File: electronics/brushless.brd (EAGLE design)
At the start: 34.3 x 56.2 mm, 63 parts, among them J1 USB_MINI-B_SMT, X1 JST-XH-10-PIN-LONG-PAD

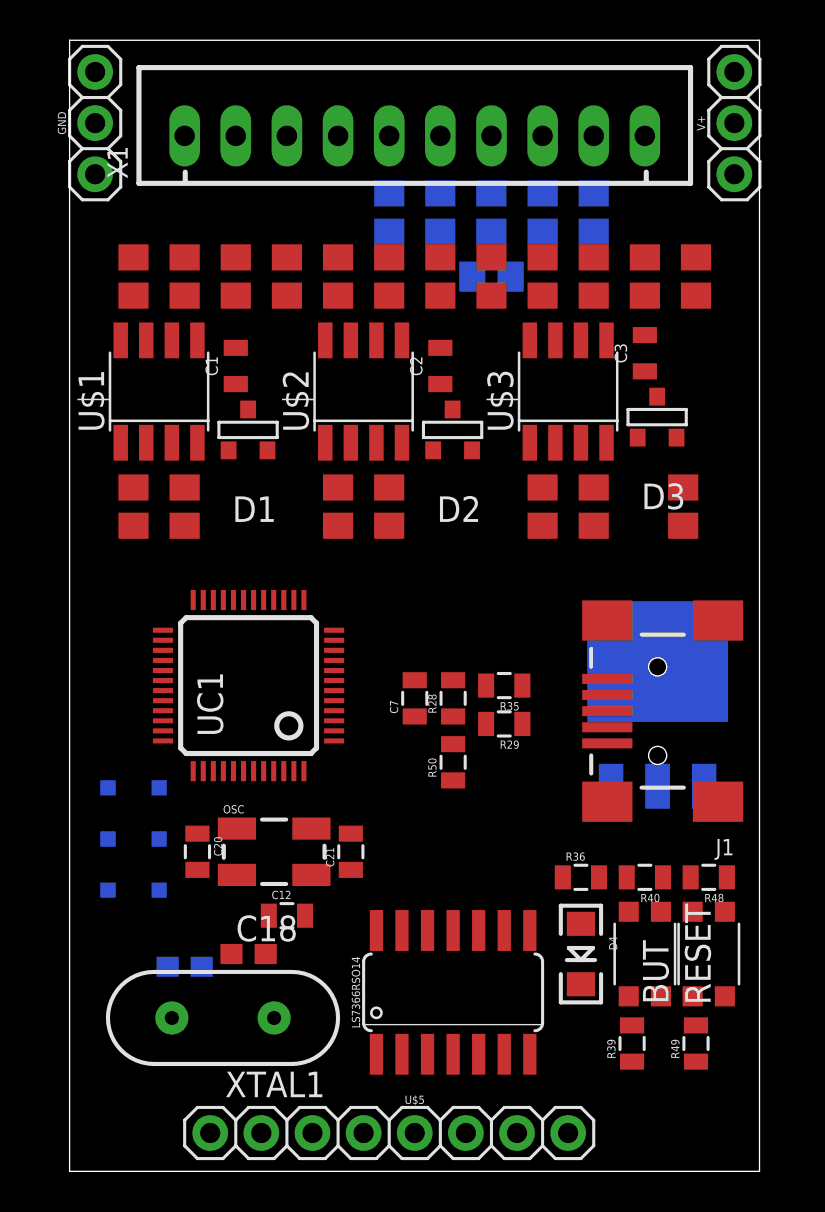
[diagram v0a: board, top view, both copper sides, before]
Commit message: mos (wip)
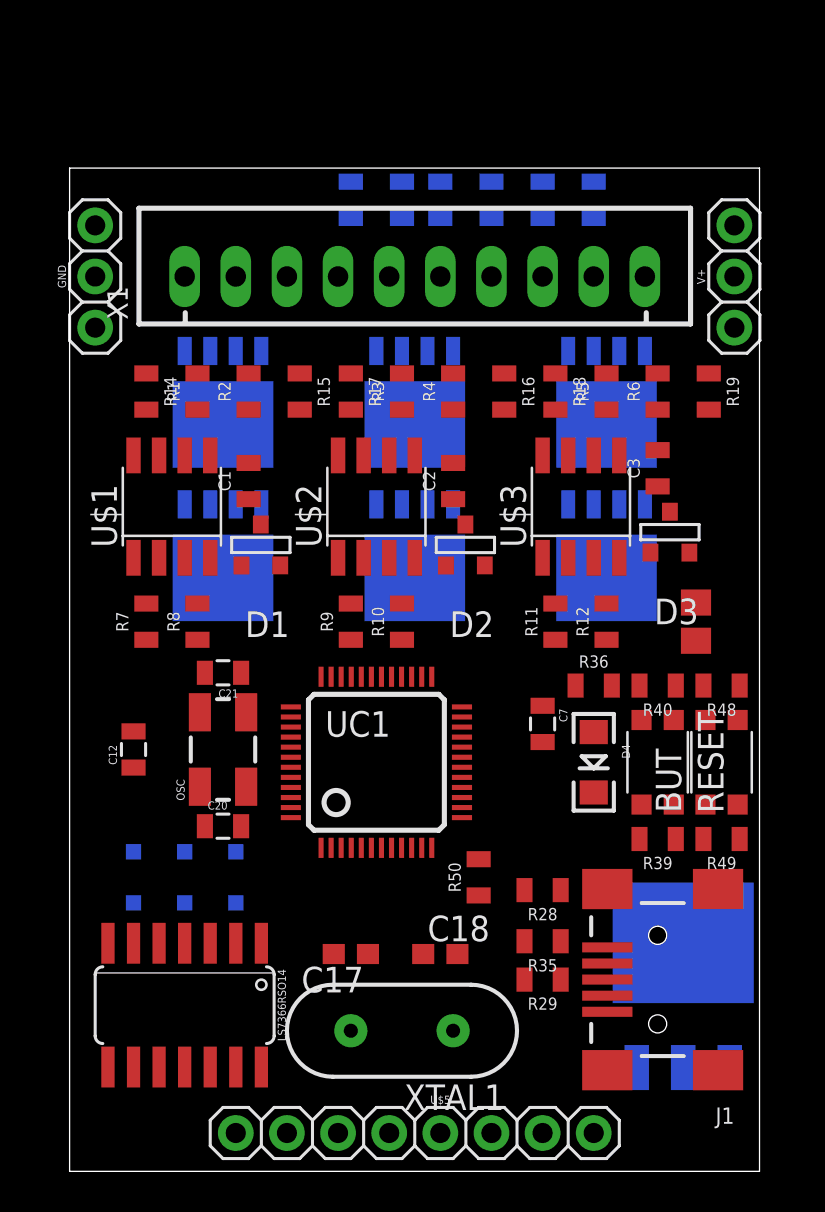
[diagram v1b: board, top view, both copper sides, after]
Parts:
- added Q1, Q2, Q3, Q4, Q5, Q6: BUK7Y12-40E, transistor-power:SOT669
- R1, R10, R11, R12, R14, R15, R16, R17, R18, R19, R2, R20, R21, R22, R23, R24, R25, R3, R4, R5, R6, R7, R8, R9: device rhoban:R0805 -> SparkFun-Resistors:0805
- R28, R29, R35, R36, R39, R40, R48, R49, R50: device SparkFun-Passives:0805 -> SparkFun-Resistors:0805
- moved U$4 14.0 mm to (30.5, 8.26)
- moved ENC1 13.4 mm to (5.71, 8.26), turned to 180 degrees
- moved J1 13.3 mm to (29.2, 9.53)
- moved R29 12.8 mm to (23.5, 9.53)
- moved R35 12.8 mm to (23.5, 11.4)
- moved C12 11.2 mm to (3.17, 21.0), turned to 90 degrees
- moved C21 10.9 mm to (7.62, 24.8), turned to 180 degrees
- moved R28 10.5 mm to (23.5, 14.0), turned to 180 degrees
- moved R39 10.2 mm to (29.2, 16.5), turned to 180 degrees
- moved R49 10.2 mm to (32.4, 16.5), turned to 180 degrees
- moved BUT 9.55 mm to (32.4, 20.3)
- moved D4 9.55 mm to (26.0, 20.3)
- moved RESET 9.55 mm to (29.2, 20.3)
- moved R36 9.55 mm to (26.0, 24.1)
- moved R40 9.55 mm to (29.2, 24.1)
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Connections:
- net GND: now also Q2.1, Q2.2, Q2.3, Q4.1, Q4.2, Q4.3, Q6.1, Q6.2, Q6.3
- net N$1: now also Q1.4
- net N$2: now also Q3.4
- net N$3: now also Q2.4
- net N$6: now also Q4.4
- net N$7: now also Q5.4
- net N$9: now also Q6.4
- net U_PHASE: now also Q1.1, Q1.2, Q1.3, Q2.MB
- net V+: now also Q1.MB, Q3.MB, Q5.MB
- net V_PHASE: now also Q3.1, Q3.2, Q3.3, Q4.MB
- net W_PHASE: now also Q5.1, Q5.2, Q5.3, Q6.MB
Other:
- board size 34.3 x 56.2 mm -> 34.3 x 49.8 mm

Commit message: tweak
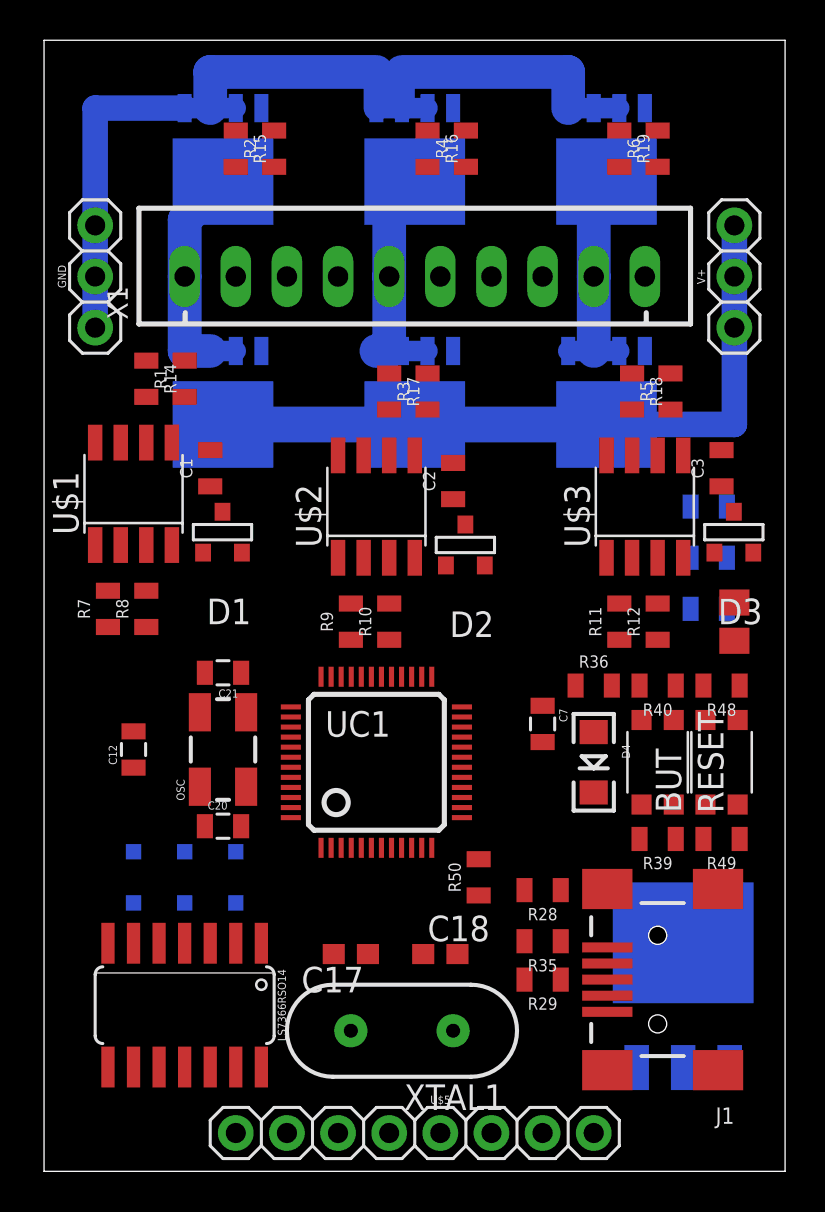
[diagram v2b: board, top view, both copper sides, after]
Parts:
- removed R20, R21, R22: 2K, SparkFun-Resistors:0805
- R23, R24, R25: value 3K -> 15K
- moved R23 25.4 mm to (31.8, 27.9), turned to 180 degrees
- moved R24 25.1 mm to (31.8, 30.5), turned to 180 degrees
- moved Q2 19.7 mm to (7.62, 50.2)
- moved Q4 19.7 mm to (17.1, 50.2)
- moved Q6 19.7 mm to (26.7, 50.2)
- moved R25 16.3 mm to (31.8, 33.0), turned to 180 degrees
- moved R19 12.9 mm to (27.3, 50.8)
- moved R16 12.7 mm to (17.8, 50.8)
- moved R15 12.5 mm to (8.26, 50.8)
- moved R2 12.1 mm to (10.2, 50.8)
- moved R4 12.1 mm to (19.7, 50.8)
- moved R6 12.1 mm to (29.2, 50.8)
- moved R18 3.81 mm to (27.9, 38.7)
- moved D3 3.18 mm to (33.0, 31.8)
- moved R11 3.18 mm to (27.3, 27.3)
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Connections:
- removed net HALL1: R20.2, X1.6
- removed net HALL2: R21.2, X1.7
- removed net HALL3: R22.2, X1.8
- net ENC_A: now also X1.3; no longer X1.9
- net ENC_B: now also X1.4; no longer X1.10
- net GND: now also X1.10; no longer X1.4
- net HALLU: now also X1.6; no longer R20.1
- net HALLV: now also X1.7; no longer R21.1
- net HALLW: now also X1.8; no longer R22.1
- net VCC: now also X1.2; no longer X1.5
- net V_PHASE: now also X1.5; no longer X1.2
- net W_PHASE: now also X1.9; no longer X1.3
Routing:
- net GND: track 0.00 -> 46.7 mm
- net V+: track 0.00 -> 35.3 mm
- net U_PHASE: track 0.00 -> 11.7 mm
- net V_PHASE: track 0.00 -> 11.5 mm
- net W_PHASE: track 0.00 -> 11.2 mm
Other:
- board size 34.3 x 49.8 mm -> 36.8 x 56.2 mm
